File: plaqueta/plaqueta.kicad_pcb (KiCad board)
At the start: 2 copper layers, 49 x 76 mm, 3 parts, among them J1 Conn_01x08_Female, J2 Conn_01x04_Female, U1 ESP32_DevKit_V1_DOIT

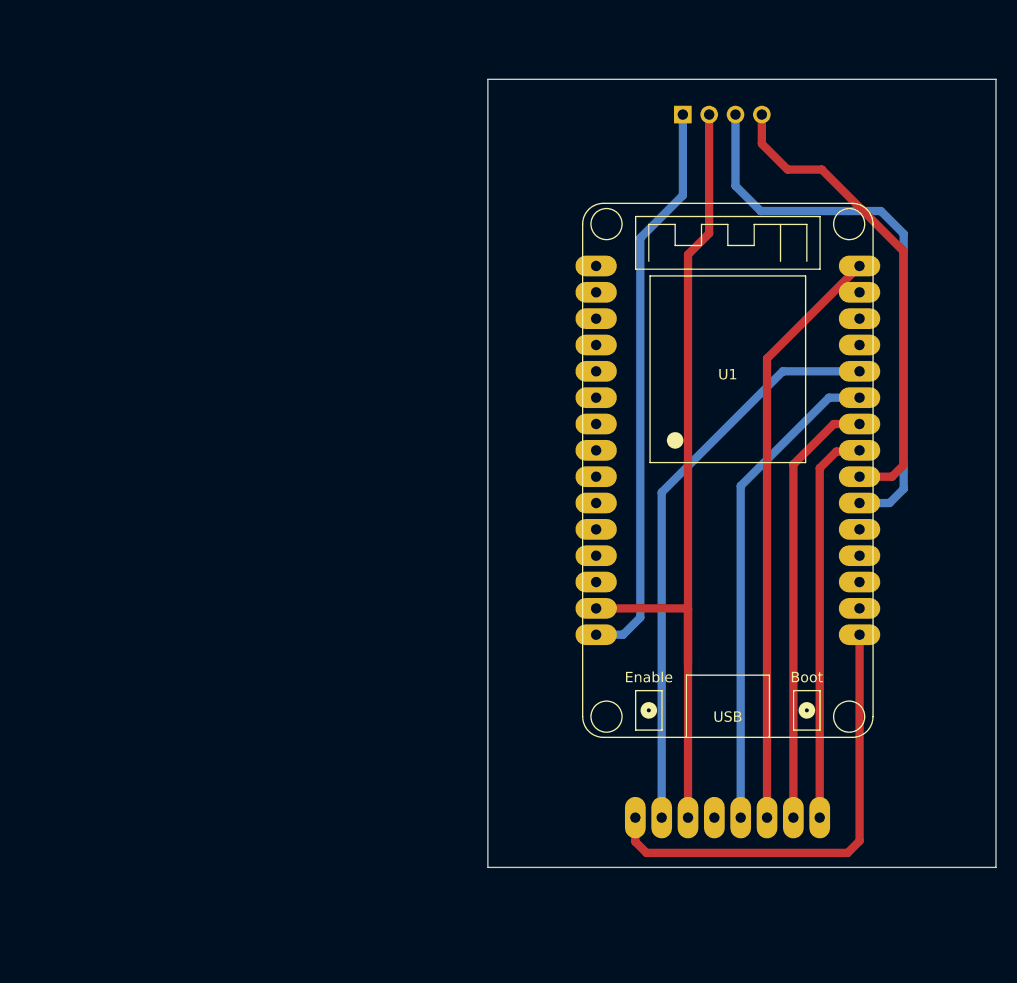
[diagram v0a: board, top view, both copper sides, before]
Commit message: updates for eb
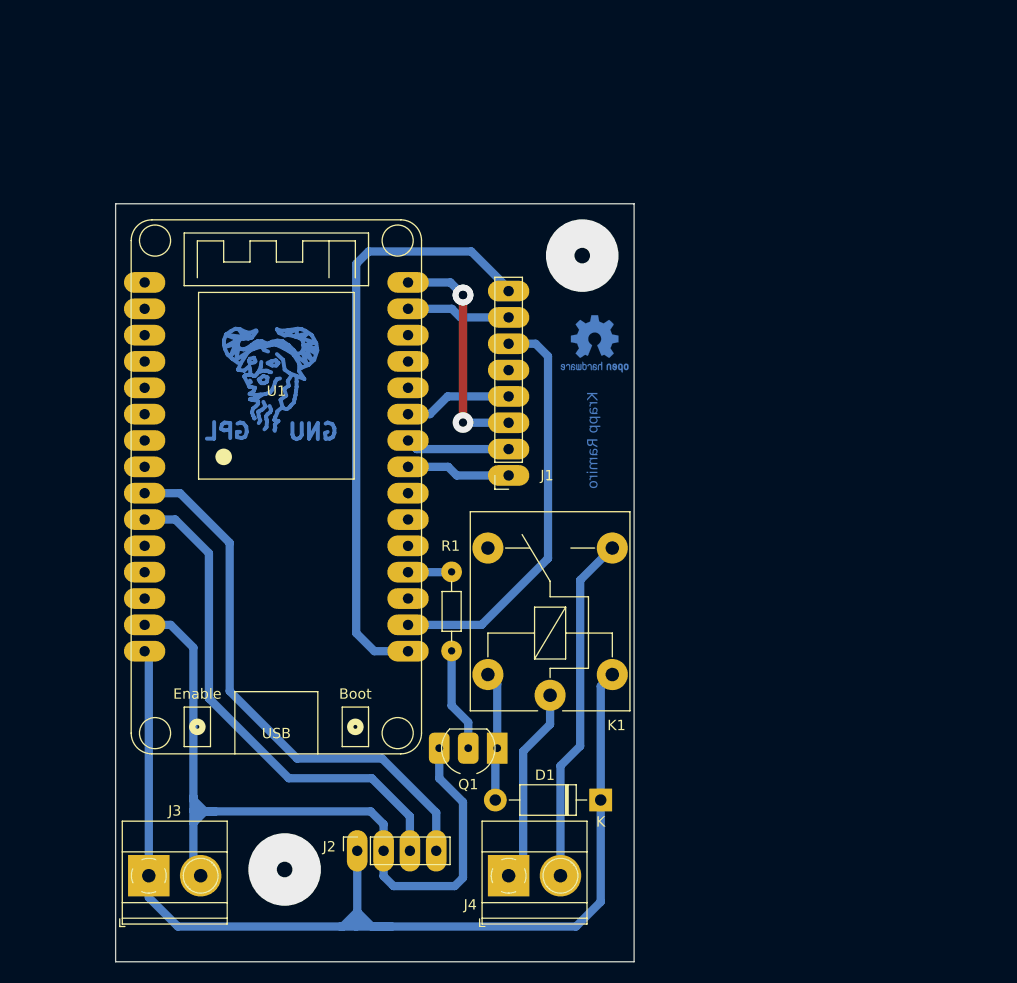
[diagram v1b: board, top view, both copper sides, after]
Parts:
- added D1: 1N4007, Diode_THT:D_DO-41_SOD81_P10.16mm_Horizontal, F.Cu at (136.9, 150.9)
- added J3: POWER, kicad_user_libraries:tblock_2x1, F.Cu at (93.3, 158.2)
- added J4: BORN_RELAY, kicad_user_libraries:tblock_2x1, F.Cu at (128.0, 158.2)
- added K1: FINDER-36.11, Relay_THT:Relay_SPDT_Finder_36.11, F.Cu at (132.0, 140.8)
- added Q1: BC337, kicad_user_libraries:krapp-TO-92_HandSolder, F.Cu at (125.4, 145.9)
- added R1: 10k, kicad_user_libraries:krapp-res-generic, F.Cu at (122.5, 128.9)
- added REF**: OSHW-Logo2_7.3x6mm_Copper, Symbol:OSHW-Logo2_7.3x6mm_Copper, B.Cu at (136.3, 106.9)
- added REF**: Symbol_GNU-Logo_CopperTop, Symbol:Symbol_GNU-Logo_CopperTop, B.Cu at (104.8, 109.2)
- J1: moved to F.Cu
- J2: footprint Connector_PinHeader_2.54mm:PinHeader_1x04_P2.54mm_Vertical -> Connector_PinSocket_2.54mm:PinSocket_1x04_P2.54mm_Vertical; moved to F.Cu
- moved J2 77.6 mm to (113.4, 155.8), turned to 90 degrees
- moved J1 44.6 mm to (128.0, 119.6), turned to 180 degrees
- moved U1 43.6 mm to (105.6, 101.0)
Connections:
- J2 pad 3: Net-(U1-Pad21) -> /I2C_SCL
- J2 pad 4: Net-(U1-Pad22) -> /I2C_SDA
- U1 pad 10: unconnected-(U1-Pad10) -> /I2C_SCL
- U1 pad 19: unconnected-(U1-Pad19) -> Net-(U1-Pad19)
- U1 pad 21: Net-(U1-Pad21) -> unconnected-(U1-Pad21)
- U1 pad 22: Net-(U1-Pad22) -> unconnected-(U1-Pad22)
- U1 pad 26: /RST/Reset -> unconnected-(U1-Pad26)
- U1 pad 29: unconnected-(U1-Pad29) -> /RST/Reset
- U1 pad 9: unconnected-(U1-Pad9) -> /I2C_SDA
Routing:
- net Net-(U1-Pad21): track 54.4 -> 0.00 mm
- net /I2C_SDA: track 0.00 -> 52.9 mm
- net +5V: track 55.1 -> 105.5 mm
- net /I2C_SCL: track 0.00 -> 49.0 mm
- net Net-(U1-Pad22): track 46.1 -> 0.00 mm
- net /RST/Reset: track 53.7 -> 10.0 mm
- net GND: track 81.3 -> 118.0 mm
- net /SPI MISO: track 45.4 -> 10.4 mm
- net Net-(J4-Pad2): track 0.00 -> 33.7 mm
- net /SPI MOSI: track 55.3 -> 22.3 mm, vias 0 -> 3
- net /SPI SCK: track 40.5 -> 8.44 mm
- net /SPI SS: track 36.7 -> 10.0 mm
- net Net-(J4-Pad1): track 0.00 -> 19.1 mm
- net Net-(D1-Pad2): track 0.00 -> 12.5 mm
- net +3.3V: track 46.4 -> 58.2 mm
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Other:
- board size 49 x 76 mm -> 50 x 73.1 mm
- board text added: "Krapp Ramiro"

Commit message: actualizado el informe
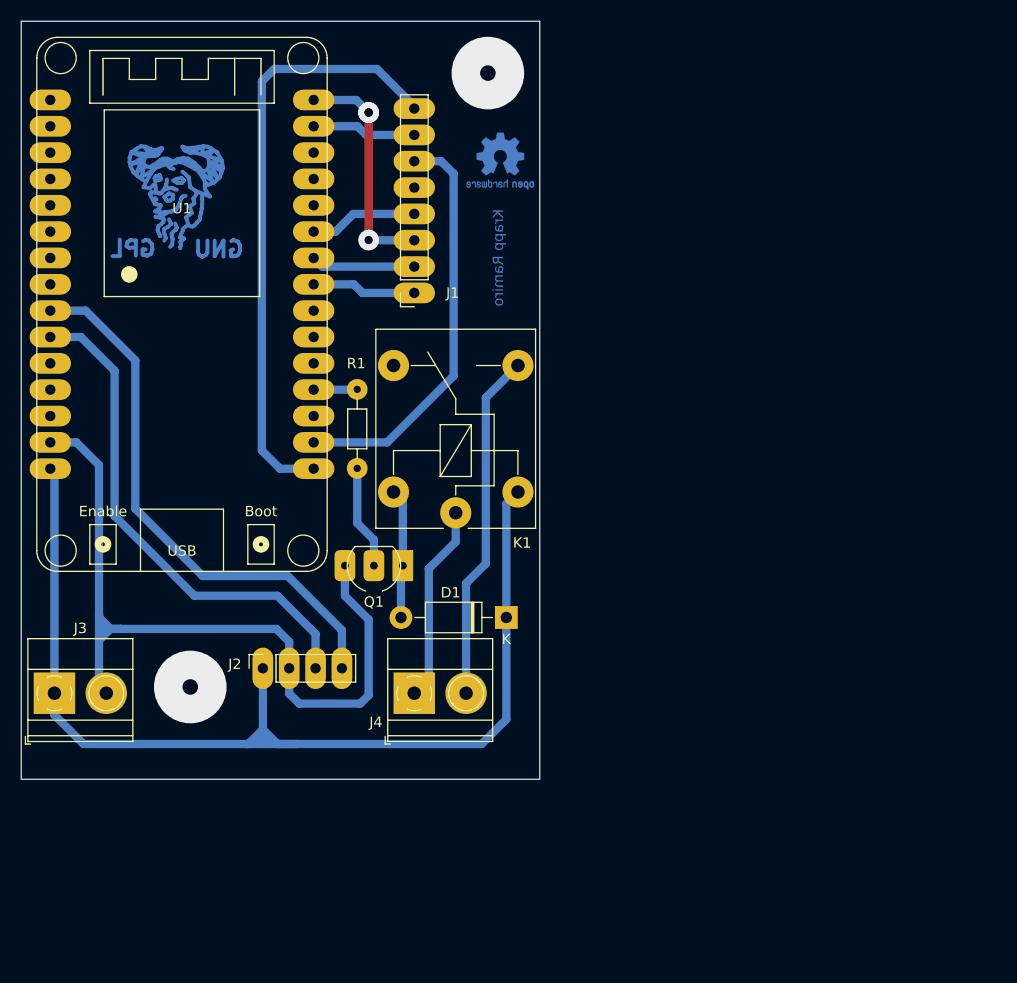
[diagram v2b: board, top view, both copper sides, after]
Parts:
- moved J2 19.8 mm to (104.3, 138.2)
- moved REF** 19.8 mm to (127.2, 89.3)
- moved K1 19.8 mm to (122.9, 123.2)
- moved R1 19.8 mm to (113.4, 111.3)
- moved REF** 19.8 mm to (95.7, 91.6)
- moved Q1 19.8 mm to (116.3, 128.3)
- moved D1 19.8 mm to (127.8, 133.3)
- moved J1 19.8 mm to (118.9, 102.0)
- moved J3 19.8 mm to (84.2, 140.6)
- moved J4 19.8 mm to (118.9, 140.6)
- moved U1 19.8 mm to (96.5, 83.4)
